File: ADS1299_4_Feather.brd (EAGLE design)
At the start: 100 x 50 mm, 40 parts, among them U1 ADS1299-4PAG

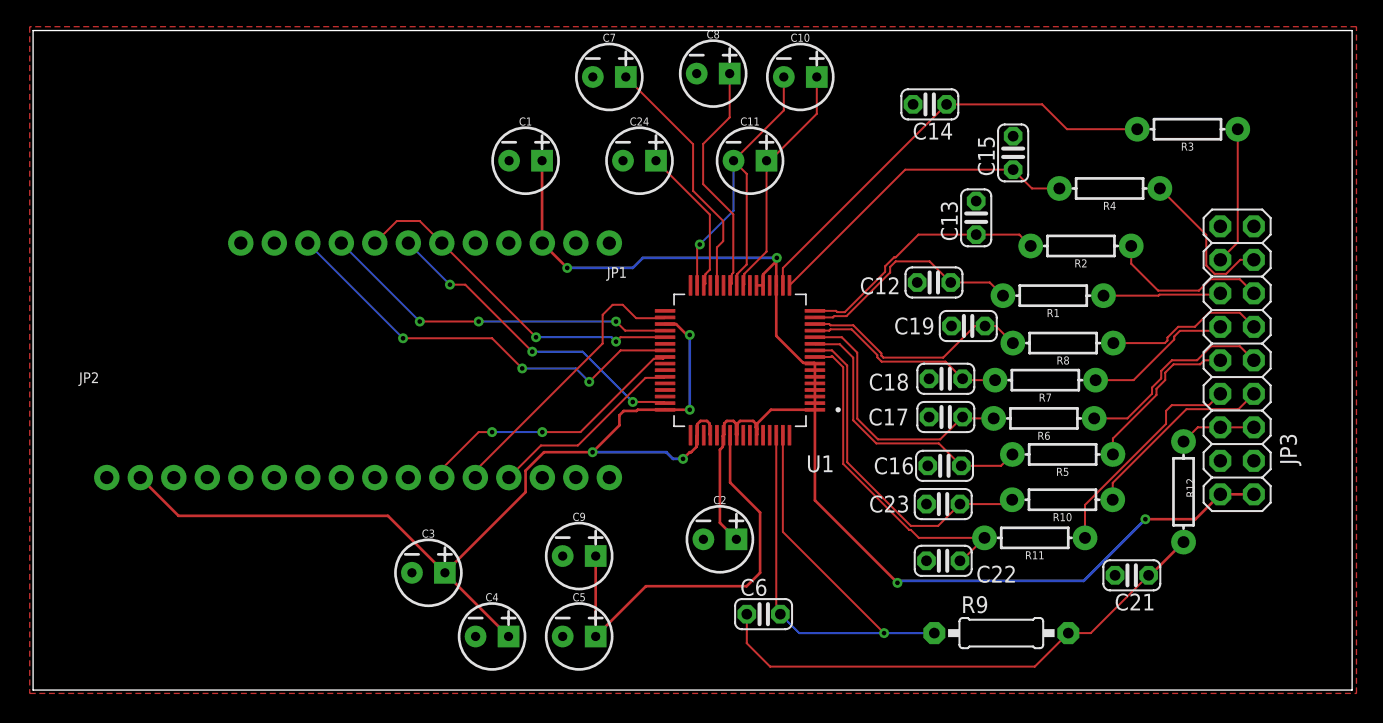
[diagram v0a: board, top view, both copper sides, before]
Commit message: modified:   ADS1299_4_Feather.brd 	modified:   ADS1299_4_Feather.sch
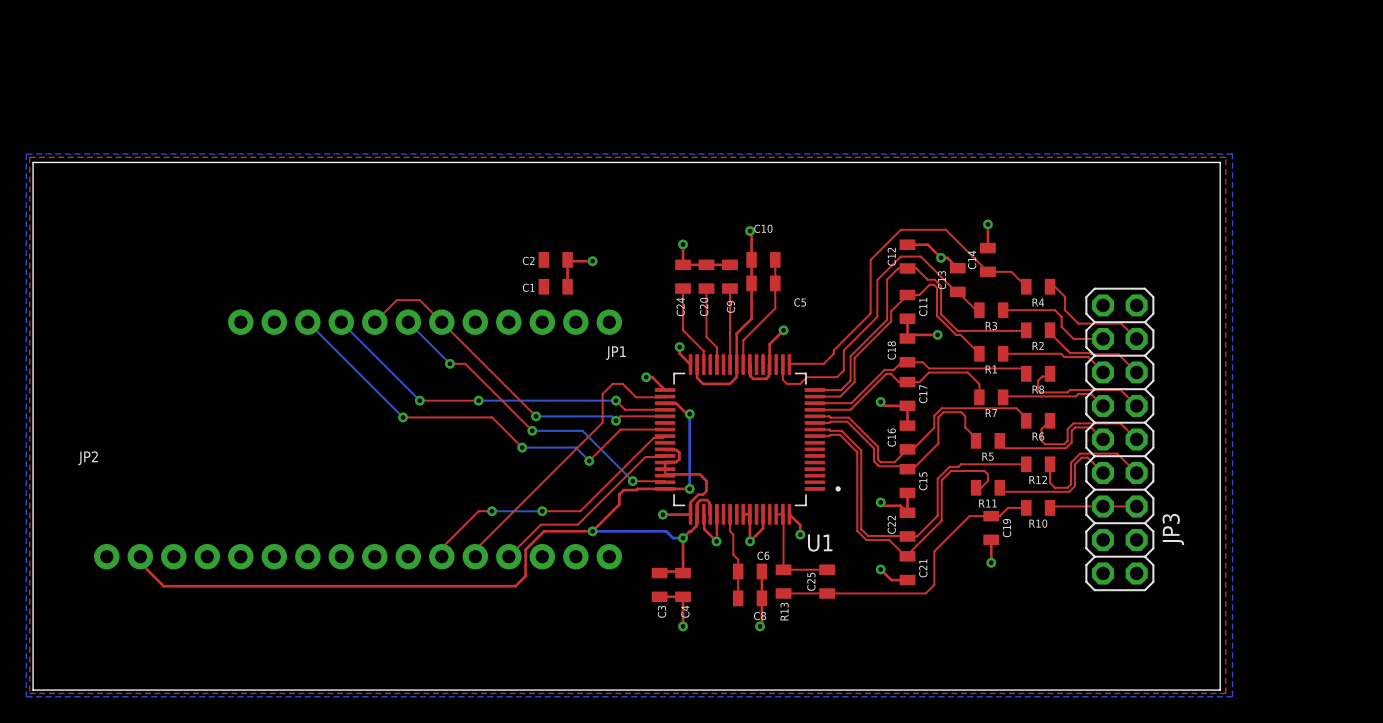
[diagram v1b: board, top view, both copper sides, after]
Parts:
- removed C23: 1 nF, adafruit:C025-024X044
- removed C7: 100uF, SparkFun-Capacitors:CPOL-RADIAL-2.5MM-5MM
- removed R9: 1M, adafruit:0207/10
- added C20: 100uF, SparkFun-Capacitors:0805
- added C25: 1nF, SparkFun-Capacitors:0805
- added R13: 1M, SparkFun-Resistors:0805
- C1, C10, C2, C24, C3, C4, C5, C8, C9: device SparkFun-Capacitors:CPOL-RADIAL-2.5MM-5MM -> SparkFun-Capacitors:0805
- C11: value 0.1uF -> 1nF; device SparkFun-Capacitors:CPOL-RADIAL-2.5MM-5MM -> SparkFun-Capacitors:0805
- C12, C13, C14, C15, C16, C17, C18, C19, C21, C22: value 1 nF -> 1nF; device adafruit:C025-024X044 -> SparkFun-Capacitors:0805
- C6: value 1 nF -> 0.1uF; device adafruit:C025-024X044 -> SparkFun-Capacitors:0805
- R1, R10, R11, R12, R2, R3, R4, R5, R6, R7, R8: device SparkFun-Resistors:AXIAL-0.3 -> SparkFun-Resistors:0805
- moved C8 39.9 mm to (54.4, 6.95)
- moved C5 30.2 mm to (55.4, 30.8), turned to 180 degrees
- moved C15 26.1 mm to (66.3, 15.8), turned to 270 degrees
- moved C2 24.6 mm to (39.6, 32.6)
- moved C9 24.1 mm to (52.8, 31.3), turned to 90 degrees
- moved R3 20.2 mm to (72.6, 28.8)
- moved C3 17.6 mm to (47.5, 7.97), turned to 270 degrees
- moved C21 17.0 mm to (66.3, 9.24), turned to 270 degrees
- moved C11 16.3 mm to (66.3, 29.1), turned to 270 degrees
- moved C19 15.4 mm to (72.6, 12.3), turned to 270 degrees
- moved C4 15.0 mm to (49.3, 7.97), turned to 270 degrees
- moved C10 14.2 mm to (55.4, 32.6), turned to 180 degrees
- moved C14 12.6 mm to (72.4, 32.6), turned to 90 degrees
- moved R12 11.2 mm to (76.2, 17.1), turned to 180 degrees
- moved JP3 10.7 mm to (82.4, 19.0)
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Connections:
- removed net N$2: C10.2, C11.2, U1.25, U1.31
- net 1_N: now also R1.1; no longer R1.P$1
- net 1_P: now also R2.1; no longer R2.P$1
- net 2_N: now also R7.1; no longer R7.P$1
- net 2_P: now also R8.1; no longer R8.P$1
- net 3_N: now also R5.1; no longer R5.P$1
- net 3_P: now also R6.1; no longer R6.P$1
- net 4_N: now also R11.1; no longer R11.P$1
- net 4_P: now also R12.1; no longer R10.P$1
- net BIAS: now also R10.1; no longer R12.P$1
- net BIAS_DRV: now also C19.1, C25.1, R10.2, R13.1; no longer C21.1, C6.1, R12.P$2, R9.2
- net BIAS_IN: now also C25.2, R13.2; no longer C6.2, R9.1
- net GND: now also C10.2, C11.2, C20.2, C6.2, U1.25, U1.31; no longer C23.2, C7.2
- net IN1_N: now also C11.1, R1.2; no longer C12.1, R1.P$2
- net IN1_P: now also C12.1, R2.2; no longer C13.1, R2.P$2
- net IN2_N: now also C17.1, R7.2; no longer C18.1, R7.P$2
- net IN2_P: now also C18.1, R8.2; no longer C19.1, R8.P$2
- net IN3_N: now also C15.1, R5.2; no longer C16.1, R5.P$2
- net IN3_P: now also C16.1, R6.2; no longer C17.1, R6.P$2
- net IN4_N: now also C21.1, R11.2; no longer C22.1, R11.P$2
- net IN4_P: now also C22.1, R12.2; no longer C23.1, R10.P$2
- net N$1: now also C5.1; no longer C11.1
- net N$4: now also C6.1, C8.1; no longer C5.1, C9.1
- net N$5: now also C20.1; no longer C7.1
- net N$6: now also C9.1; no longer C8.1
- net SRB1: now also R4.1; no longer R4.P$1
- net SRB2: now also R3.1; no longer R3.P$1
- net _SRB1: now also C14.1, R4.2; no longer C15.1, R4.P$2
- net _SRB2: now also C13.1, R3.2; no longer C14.1, R3.P$2
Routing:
- net 5V: track 106.9 -> 0.00 mm, vias 4 -> 0
- net GND: track 0.00 -> 89.0 mm, vias 0 -> 19
- net BIAS_IN: track 44.1 -> 8.02 mm, vias 1 -> 0
- net N$2: track 28.7 -> 0.00 mm, vias 1 -> 0
- net N$4: track 31.9 -> 6.62 mm
- net BIAS_DRV: track 40.0 -> 22.6 mm
- net N$5: track 19.1 -> 6.09 mm
- net N$6: track 17.9 -> 5.76 mm
- net _SRB2: track 34.1 -> 24.4 mm
- net N$1: track 18.4 -> 8.93 mm
- net IN1_P: track 19.4 -> 25.9 mm
- net 4_N: track 16.8 -> 10.5 mm
- net 3V3: track 78.1 -> 72.1 mm
- net N$3: track 11.3 -> 6.41 mm
- net 3_P: track 15.4 -> 10.8 mm
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- added copper zone on layer 1, net 5V
- added copper zone on layer 16, net GND
- removed copper zone on layer 1, net GND
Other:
- board size 100 x 50 mm -> 90 x 40 mm
